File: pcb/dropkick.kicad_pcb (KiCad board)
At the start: 2 copper layers, 44.5 x 50.8 mm, 51 parts, among them SW1 CONN3_020524_WRE, SW2 KMR211NG_LFS, U1 ATSAMD21G18A-AUT, U2 SAM-M8Q-0-10, U3 MCP73831T-2ACI/OT, U4 DPS310, U5 MPU-6050, U6 SPX3819-3.3, X1 microUSB, X2 JSTPH, X3 microsd, X5 32768Hz

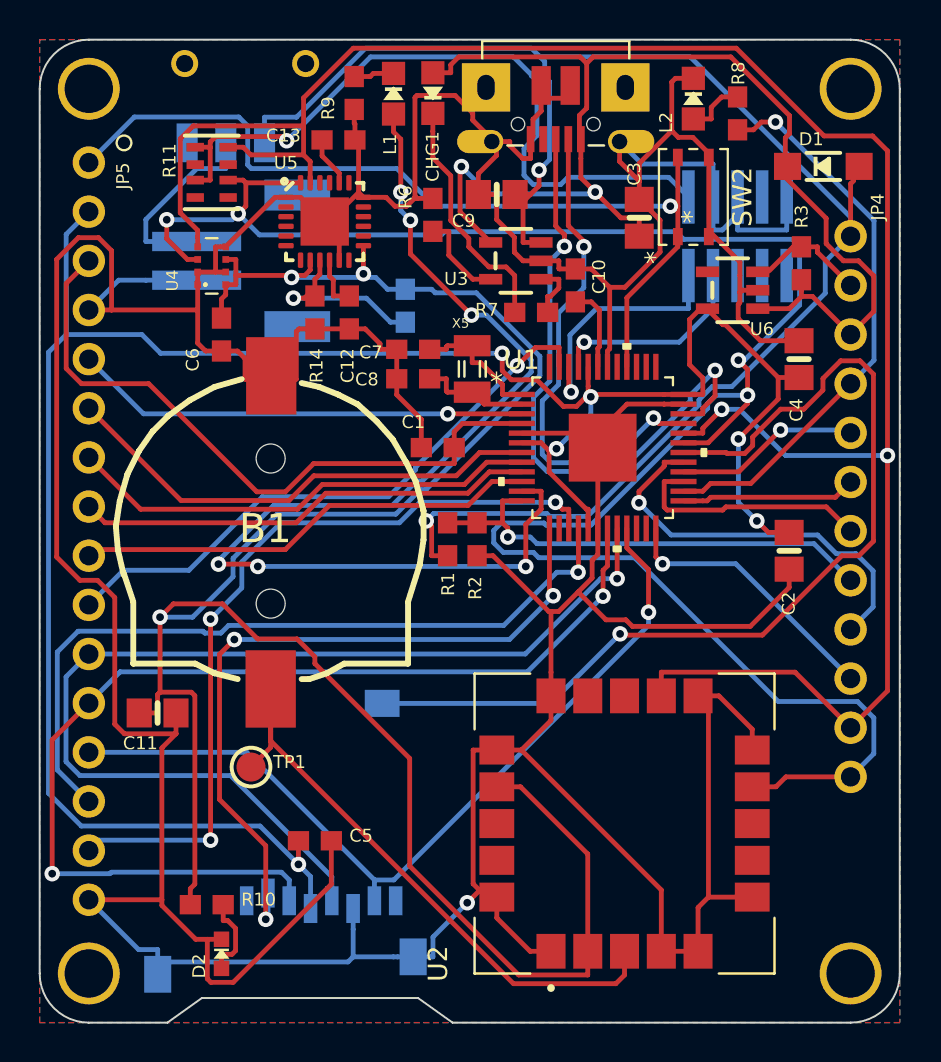
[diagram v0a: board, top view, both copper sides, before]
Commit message: V3 board
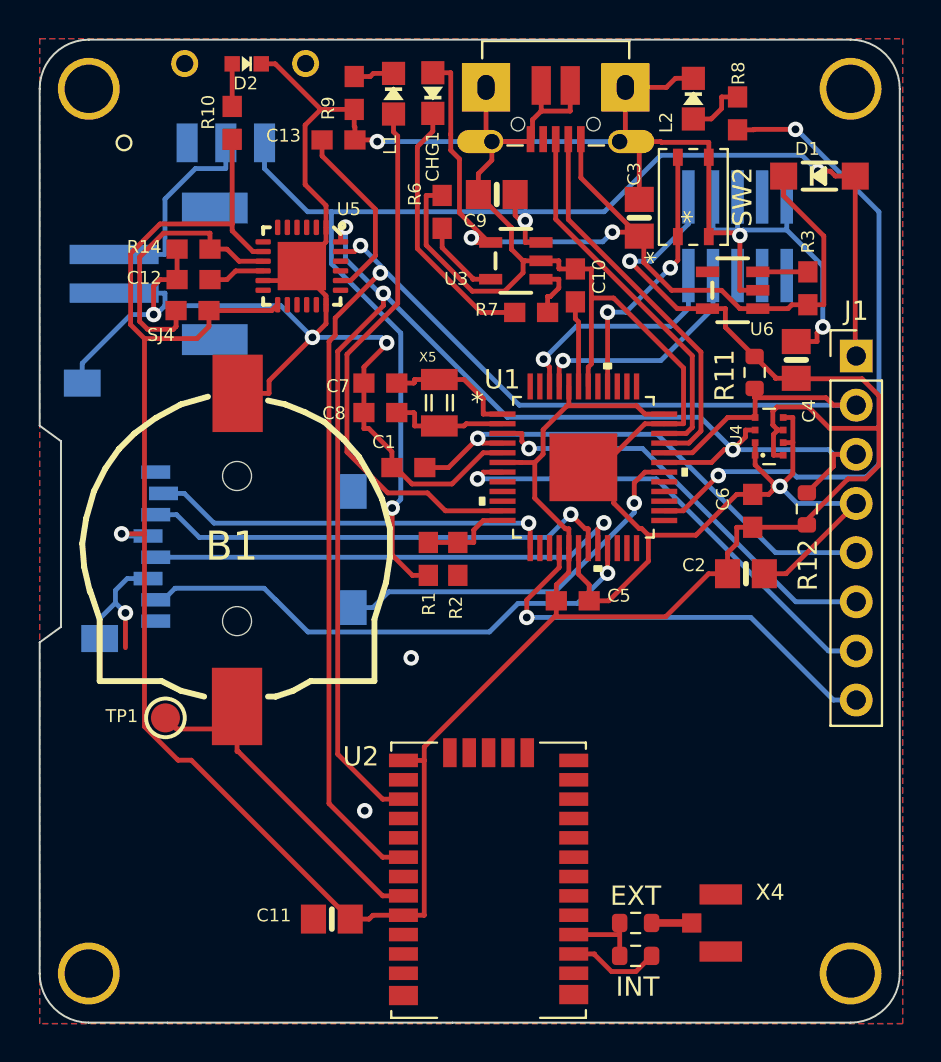
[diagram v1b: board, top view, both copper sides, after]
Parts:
- removed JP4: HEADER-1X12, lib_fr:1X12_ROUND
- removed JP5: HEADER-1X16ROUND, lib_fr:1X16_ROUND
- added J1: Conn_01x08, Connector_PinHeader_2.54mm:PinHeader_1x08_P2.54mm_Vertical, F.Cu at (105.7, 60.8)
- added R12: 10K, Resistor_SMD:R_0603_1608Metric, F.Cu at (103.2, 68.7)
- added R4: 0K, Resistor_SMD:R_0603_1608Metric, F.Cu at (94.3, 91.8)
- added R5: 0K, Resistor_SMD:R_0603_1608Metric, F.Cu at (94.3, 90.1)
- added X4: ANTENNA_U.FL, lib_fr:U.FL, F.Cu at (98.7, 90.1)
- JP2: value 20021221-00010C4LF -> 3221-10-0300-00-TR
- R11: value 4.7K -> 10K; footprint lib_fr:RESPACK_4X0603 -> Resistor_SMD:R_0603_1608Metric
- SJ4: moved to F.Cu
- SW1: value CONN3_020524_WRE -> 450405020524
- U2: value SAM-M8Q-0-10 -> QFN_M8C-0_UBL; footprint lib_fr:MODULE_SAM-M8Q-0-10 -> lib_fr:CAM-M8C-0
- U4: value DPS310 -> DPS310XTSA1
- moved D2 46.0 mm to (74.2, 45.7), turned to -90 degrees
- moved R10 40.4 mm to (73.5, 48.8), turned to 90 degrees
- moved U4 30.1 mm to (101.2, 65.0)
- moved R11 29.9 mm to (100.5, 61.6)
- moved C6 28.9 mm to (100.3, 68.8), turned to 90 degrees
- moved C5 18.2 mm to (91.0, 73.5)
- moved C11 13.9 mm to (78.6, 89.9), turned to 180 degrees
- moved REF** 11.3 mm to (90.2, 73.7)
- moved SJ4 11.0 mm to (71.4, 58.5), turned to 180 degrees
- moved C12 8.23 mm to (71.5, 56.9), turned to 180 degrees
- moved U2 7.54 mm to (86.7, 87.7), turned to 180 degrees
- moved R14 7.07 mm to (71.5, 55.3), turned to 180 degrees
- moved TP1 5.10 mm to (70.0, 79.5)
- moved X2 4.32 mm to (71.0, 56.5)
- moved X3 3.96 mm to (80.1, 75.8), turned to 90 degrees
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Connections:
- C11 pad 1: 3.3V -> +3V3
- C6 pad 1: 3.3V -> +3V3
- JP2 pad 1: VCC -> +3V3
- R10 pad 1: 3.3V -> +3V3
- R11 pad 1: VCC -> +3V3
- R11 pad 2: (no net) -> /SCL
- SJ4 pad 1: 3.3V -> +3V3
- U2 pad 1: GND -> +3V3
- U2 pad 12: /SCL -> GND
- U2 pad 13: unconnected-(U2-Pad13) -> GND
- U2 pad 14: unconnected-(U2-Pad14) -> GND
- U2 pad 16: GND -> /RF
- U2 pad 17: 3.3V -> Net-(R4-Pad2)
- U2 pad 18: unconnected-(U2-Pad18) -> GND
- U2 pad 19: unconnected-(U2-Pad19) -> GND
- U2 pad 2: 3.3V -> unconnected-(U2-Pad2)
- U2 pad 20: GND -> unconnected-(U2-Pad20)
- U2 pad 3: /VBACKUP -> /SDA
- U2 pad 6: GND -> /SCL
- U2 pad 8: unconnected-(U2-Pad8) -> /VBACKUP
- U2 pad 9: /SDA -> +3V3
- U4 pad 6: 3.3V -> +3V3
- U4 pad 8: 3.3V -> +3V3
- U5 pad 13: 3.3V -> +3V3
- U5 pad 8: 3.3V -> +3V3
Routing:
- net GND: track 337.6 -> 219.5 mm, vias 1 -> 10
- net 3.3V: track 116.2 -> 0.00 mm, vias 3 -> 0
- net +3V3: track 118.3 -> 161.6 mm, vias 6 -> 2
- net /D1: track 40.9 -> 0.00 mm, vias 3 -> 0
- net VCC: track 37.4 -> 0.00 mm, vias 1 -> 0
- net /SDA: track 105.4 -> 71.6 mm, vias 4 -> 3
- net /SCL: track 109.6 -> 76.3 mm
- net /~{RESET}: track 46.6 -> 13.9 mm, vias 1 -> 2
- net /MOSI: track 55.6 -> 24.6 mm, vias 2 -> 1
- net /A5: track 30.9 -> 0.00 mm, vias 1 -> 0
- net /D7: track 50.3 -> 19.9 mm
- net /D8: track 58.3 -> 27.9 mm, vias 6 -> 0
- net /SCK: track 55.0 -> 25.3 mm
- net /A2: track 24.5 -> 0.00 mm
- net /A4: track 24.0 -> 0.00 mm
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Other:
- outline, holes or cut-outs redrawn
- board text added: "A0"
- board text added: "A1"
- board text added: "AREF"
- board text added: "D0"
- board text added: "Dropkick V3 Copyright (c) 2022 Riley Rainey https://GitHub.com/rrainey/dropkick/"
- board text added: "EXT"
- board text added: "GND"
- board text added: "INT"
- board text added: "SCL"
- board text added: "SDA"
- board text added: "VBAT"
- board text removed: "Dropkick V1 Copyright (c) 2022 Riley Rainey https://GitHub.com/rrainey/dropkick/"
